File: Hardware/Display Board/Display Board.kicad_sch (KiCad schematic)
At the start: 20 parts, among them J1 GPS, J2 RTC, J3 CONT, J4 H:M, J5 M:D, J6 M:S, J7 D:Y

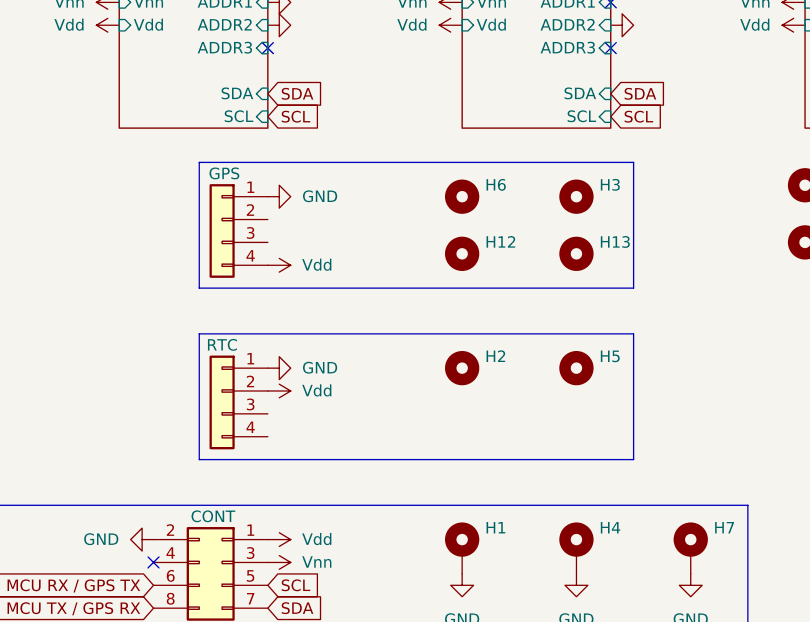
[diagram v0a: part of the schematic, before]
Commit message: Components placed
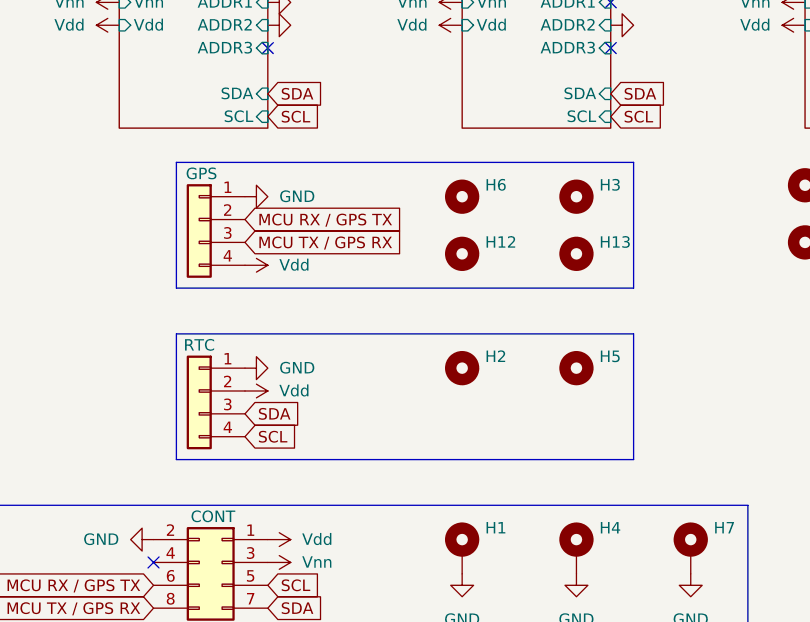
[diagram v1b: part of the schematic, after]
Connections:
- net MCU RX / GPS TX: now also J1.2 (Pin_2)
- net MCU TX / GPS RX: now also J1.3 (Pin_3)
- net SCL: now also J2.4 (Pin_4)
- net SDA: now also J2.3 (Pin_3)
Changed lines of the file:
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@@
 	)
 	(rectangle
-		(start 46.99 73.66)
+		(start 44.45 73.66)
 		(end 95.25 87.63)
 		(stroke
@@
 	)
 	(rectangle
-		(start 46.99 92.71)
+		(start 44.45 92.71)
 		(end 95.25 106.68)
 		(stroke
@@
 		)
 	)
+	(global_label "SDA"
+		(shape input)
+		(at 52.07 101.6 0)
+		(fields_autoplaced yes)
+		(effects
+			(font
+				(size 1.27 1.27)
+			)
+			(justify left)
+		)
+		(property "Intersheetrefs" "${INTERSHEET_REFS}"
+			(at 58.6233 101.6 0)
+			(effects
+				(font
+					(size 1.27 1.27)
+				)
+				(justify left)
+				(hide yes)
+			)
+		)
+	)
 	(global_label "MCU TX {slash} GPS RX"
 		(shape input)
@@
 		)
 	)
+	(global_label "MCU TX {slash} GPS RX"
+		(shape input)
+		(at 52.07 82.55 0)
+		(fields_autoplaced yes)
+		(effects
+			(font
+				(size 1.27 1.27)
+			)
+			(justify left)
+		)
+		(property "Intersheetrefs" "${INTERSHEET_REFS}"
+			(at 72.7141 82.55 0)
+			(effects
+				(font
+					(size 1.27 1.27)
+				)
+				(justify left)
+				(hide yes)
+			)
+		)
+	)
 	(global_label "SDA"
 		(shape input)
@@
 		)
 	)
+	(global_label "MCU RX {slash} GPS TX"
+		(shape input)
+		(at 52.07 80.01 0)
+		(fields_autoplaced yes)
+		(effects
+			(font
+				(size 1.27 1.27)
+			)
+			(justify left)
+		)
+		(property "Intersheetrefs" "${INTERSHEET_REFS}"
+			(at 72.7141 80.01 0)
+			(effects
+				(font
+					(size 1.27 1.27)
+				)
+				(justify left)
+				(hide yes)
+			)
+		)
+	)
 	(global_label "SDA"
 		(shape input)
@@
 		)
 	)
+	(global_label "SCL"
+		(shape input)
+		(at 52.07 104.14 0)
+		(fields_autoplaced yes)
+		(effects
+			(font
+				(size 1.27 1.27)
+			)
+			(justify left)
+		)
+		(property "Intersheetrefs" "${INTERSHEET_REFS}"
+			(at 58.5628 104.14 0)
+			(effects
+				(font
+					(size 1.27 1.27)
+				)
+				(justify left)
+				(hide yes)
+			)
+		)
+	)
 	(global_label "SDA"
 		(shape input)
@@
 	(symbol
 		(lib_id "power:GND")
-		(at 54.61 96.52 90)
+		(at 52.07 96.52 90)
 		(unit 1)
 		(exclude_from_sim no)
@@
 		(fields_autoplaced yes)
 		(property "Reference" "#PWR015"
-			(at 60.96 96.52 0)
+			(at 58.42 96.52 0)
 			(effects
 				(font
@@
 		)
 		(property "Value" "GND"
-			(at 58.42 96.5199 90)
+			(at 55.88 96.5199 90)
 			(effects
 				(font
@@
 		)
 		(property "Footprint" ""
-			(at 54.61 96.52 0)
+			(at 52.07 96.52 0)
 			(effects
 				(font
@@
 		)
 		(property "Datasheet" ""
-			(at 54.61 96.52 0)
+			(at 52.07 96.52 0)
 			(effects
 				(font
@@
 		)
 		(property "Description" "Power symbol creates a global label with name \"GND\" , ground"
-			(at 54.61 96.52 0)
+			(at 52.07 96.52 0)
 			(effects
 				(font
@@
 	(symbol
 		(lib_id "power:+5V")
-		(at 54.61 85.09 270)
+		(at 52.07 85.09 270)
 		(unit 1)
 		(exclude_from_sim no)
@@
 		(fields_autoplaced yes)
 		(property "Reference" "#PWR014"
-			(at 50.8 85.09 0)
+			(at 48.26 85.09 0)
 			(effects
 				(font
@@
 		)
 		(property "Value" "Vdd"
-			(at 58.42 85.0899 90)
+			(at 55.88 85.0899 90)
 			(effects
 				(font
@@
 		)
 		(property "Footprint" ""
-			(at 54.61 85.09 0)
+			(at 52.07 85.09 0)
 			(effects
 				(font
@@
 		)
 		(property "Datasheet" ""
-			(at 54.61 85.09 0)
+			(at 52.07 85.09 0)
 			(effects
 				(font
@@
 		)
 		(property "Description" "Power symbol creates a global label with name \"+5V\""
-			(at 54.61 85.09 0)
+			(at 52.07 85.09 0)
 			(effects
 				(font
@@
 	(symbol
 		(lib_id "Connector_Generic:Conn_01x04")
-		(at 49.53 99.06 0)
+		(at 46.99 99.06 0)
 		(mirror y)
 		(unit 1)
@@
 		(dnp no)
 		(property "Reference" "J2"
-			(at 49.276 93.726 0)
+			(at 46.736 93.726 0)
 			(effects
 				(font
@@
 		)
 		(property "Value" "RTC"
-			(at 49.53 93.98 0)
+			(at 46.99 93.98 0)
 			(effects
 				(font
@@
 		)
 		(property "Footprint" "Connector_PinSocket_2.54mm:PinSocket_1x04_P2.54mm_Vertical"
-			(at 49.53 99.06 0)
+			(at 46.99 99.06 0)
 			(effects
 				(font
@@
 		)
 		(property "Datasheet" "~"
-			(at 49.53 99.06 0)
+			(at 46.99 99.06 0)
 			(effects
 				(font
@@
 		)
 		(property "Description" "Generic connector, single row, 01x04, script generated (kicad-library-utils/schlib/autogen/connector/)"
-			(at 49.53 99.06 0)
+			(at 46.99 99.06 0)
 			(effects
 				(font
@@
 	(symbol
 		(lib_id "power:GND")
-		(at 54.61 77.47 90)
+		(at 52.07 77.47 90)
 		(unit 1)
 		(exclude_from_sim no)
@@
 		(fields_autoplaced yes)
 		(property "Reference" "#PWR013"
-			(at 60.96 77.47 0)
+			(at 58.42 77.47 0)
 			(effects
 				(font
@@
 		)
 		(property "Value" "GND"
-			(at 58.42 77.4699 90)
+			(at 55.88 77.4699 90)
 			(effects
 				(font
@@
 		)
 		(property "Footprint" ""
-			(at 54.61 77.47 0)
+			(at 52.07 77.47 0)
 			(effects
 				(font
@@
 		)
 		(property "Datasheet" ""
-			(at 54.61 77.47 0)
+			(at 52.07 77.47 0)
 			(effects
 				(font
@@
 		)
 		(property "Description" "Power symbol creates a global label with name \"GND\" , ground"
-			(at 54.61 77.47 0)
+			(at 52.07 77.47 0)
 			(effects
 				(font
@@
 	(symbol
 		(lib_id "Connector_Generic:Conn_01x04")
-		(at 49.53 80.01 0)
+		(at 46.99 80.01 0)
 		(mirror y)
 		(unit 1)
@@
 		(dnp no)
 		(property "Reference" "J1"
-			(at 49.276 74.676 0)
+			(at 46.736 74.676 0)
 			(effects
 				(font
@@
 		)
 		(property "Value" "GPS"
-			(at 49.784 74.93 0)
+			(at 47.244 74.93 0)
 			(effects
 				(font
@@
 		)
 		(property "Footprint" "Connector_PinSocket_2.54mm:PinSocket_1x04_P2.54mm_Vertical"
-			(at 49.53 80.01 0)
+			(at 46.99 80.01 0)
 			(effects
 				(font
@@
 		)
 		(property "Datasheet" "~"
-			(at 49.53 80.01 0)
+			(at 46.99 80.01 0)
 			(effects
 				(font
@@
 		)
 		(property "Description" "Generic connector, single row, 01x04, script generated (kicad-library-utils/schlib/autogen/connector/)"
-			(at 49.53 80.01 0)
+			(at 46.99 80.01 0)
 			(effects
 				(font
@@
 	(symbol
 		(lib_id "power:+5V")
-		(at 54.61 99.06 270)
+		(at 52.07 99.06 270)
 		(unit 1)
 		(exclude_from_sim no)
@@
 		(fields_autoplaced yes)
 		(property "Reference" "#PWR016"
-			(at 50.8 99.06 0)
+			(at 48.26 99.06 0)
 			(effects
 				(font
@@
 		)
 		(property "Value" "Vdd"
-			(at 58.42 99.0599 90)
+			(at 55.88 99.0599 90)
 			(effects
 				(font
@@
 		)
 		(property "Footprint" ""
-			(at 54.61 99.06 0)
+			(at 52.07 99.06 0)
 			(effects
 				(font
@@
 		)
 		(property "Datasheet" ""
-			(at 54.61 99.06 0)
+			(at 52.07 99.06 0)
 			(effects
 				(font
@@
 		)
 		(property "Description" "Power symbol creates a global label with name \"+5V\""
-			(at 54.61 99.06 0)
+			(at 52.07 99.06 0)
 			(effects
 				(font
